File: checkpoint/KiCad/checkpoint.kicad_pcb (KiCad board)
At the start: 4 copper layers, 85.2 x 39.6 mm, 113 parts, among them J1 T0, J10 CAN_OUT, J11 BOOT, J12 Y_ENDSTOP, J13 I2C, J14 SERVO, J15 RGB, J16 SWD, J17 USB_C_Receptacle_USB2.0_16P, J18 PWR_OUT, J19 PWR_CAN_IN, J2 T1, J3 T2, J4 T3, J5 2_WIRE, J6 24_3_WIRE_A, J7 PT100, J8 23_WIRE, J9 PT100_1K, Q1 BSS138, SW1 SW_RESET, U1 MAX31865xTP, U2 SN65HVD1050D, U3 STM32G0B1CBTx, U4 USBLC6-2P6, U5 AMS1117-3.3, U6 TPS5430DDA, Y1 Crystal

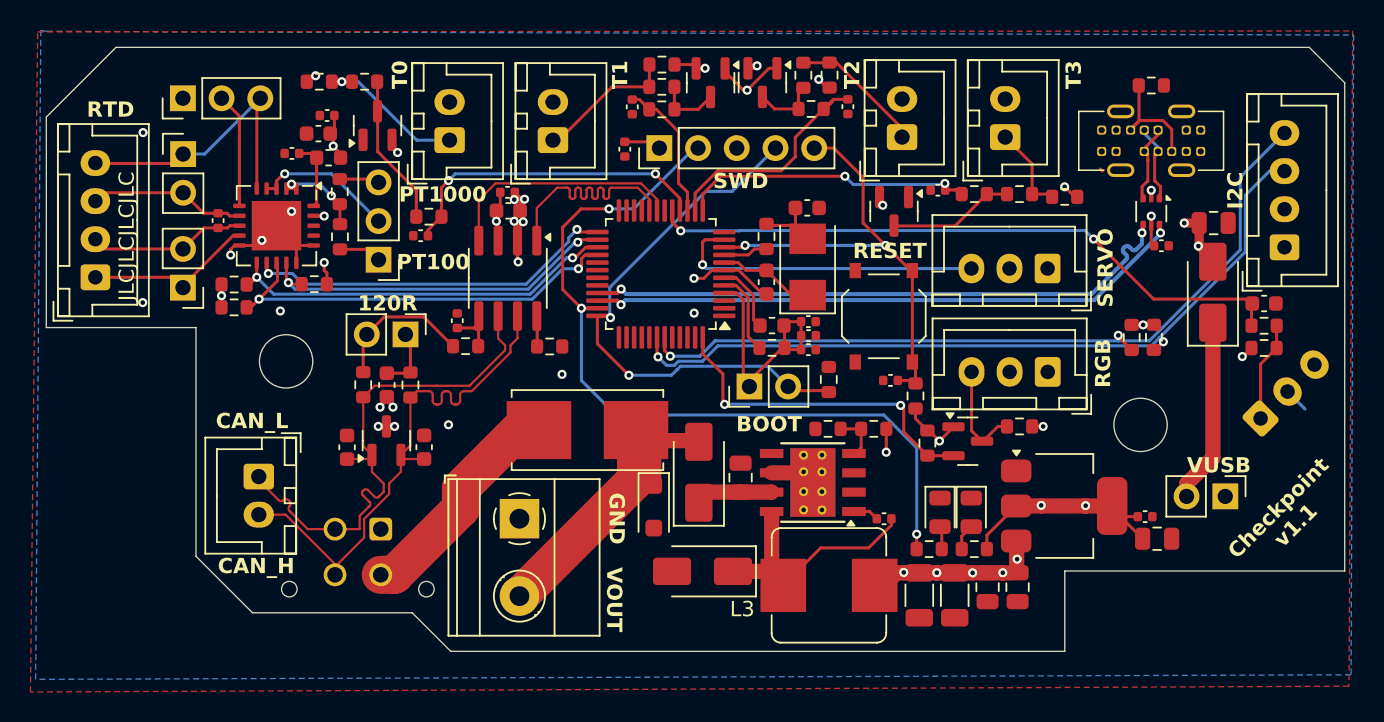
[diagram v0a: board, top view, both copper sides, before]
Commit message: chore: clean up tracks
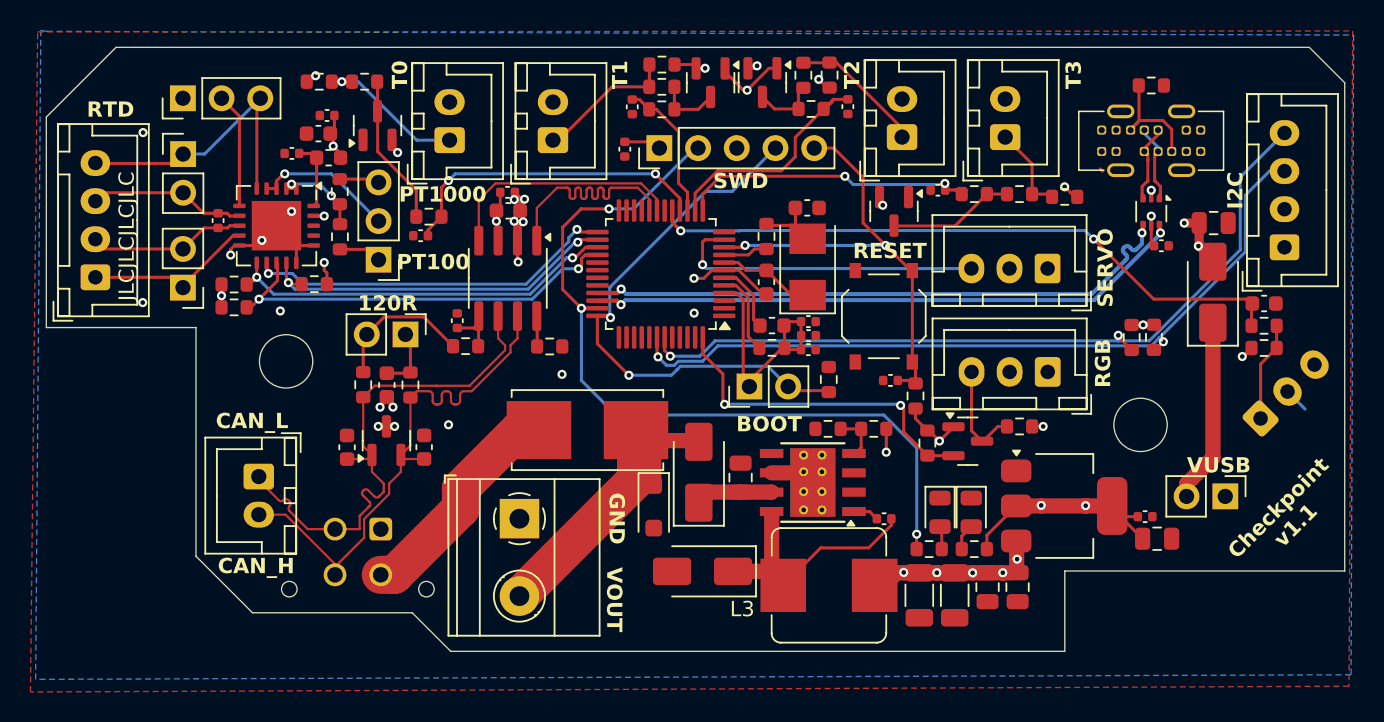
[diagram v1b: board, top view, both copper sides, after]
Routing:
- net +3.3V: track 120.7 -> 117.9 mm
- net Net-(D11-K): track 18.1 -> 15.8 mm
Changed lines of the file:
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@@
 	)
 	(segment
-		(start 44.5 57.27071)
-		(end 44.900408 57.671118)
-		(width 0.2)
-		(layer "F.Cu")
-		(net 2)
-	)
-	(segment
 		(start 53.075408 48.096118)
 		(end 53.075408 46.746118)
@@
 	)
 	(segment
+		(start 44.5 56.995)
+		(end 44.5 57.27071)
+		(width 0.2)
+		(layer "F.Cu")
+		(net 2)
+	)
+	(segment
 		(start 52.97 45.361526)
 		(end 52.97 45.066801)
@@
 	)
 	(segment
-		(start 44.5 56.995)
-		(end 44.5 57.27071)
-		(width 0.2)
-		(layer "F.Cu")
-		(net 2)
-	)
-	(segment
 		(start 53.075408 45.864592)
 		(end 53.075408 46.746118)
@@
 		(net 2)
 	)
+	(segment
+		(start 44.5 57.27071)
+		(end 44.900408 57.671118)
+		(width 0.2)
+		(layer "F.Cu")
+		(net 2)
+	)
 	(via
 		(at 34.25 47.69)
@@
 	)
 	(segment
-		(start 92.920408 65.121118)
-		(end 92.920408 63.751118)
-		(width 0.2)
-		(layer "F.Cu")
-		(net 6)
-	)
-	(segment
 		(start 85.81 64.16)
 		(end 87.411526 64.16)
@@
 	)
 	(segment
-		(start 39.440408 36.311118)
-		(end 39.245408 36.311118)
-		(width 0.2)
-		(layer "F.Cu")
-		(net 6)
-	)
-	(segment
 		(start 45.014187 40.764897)
 		(end 45.014187 40.125926)
@@
 	)
 	(segment
-		(start 89.650408 43.871118)
-		(end 89.815408 43.871118)
-		(width 0.2)
-		(layer "F.Cu")
-		(net 6)
-	)
-	(segment
 		(start 40.390408 48.691118)
 		(end 40.565408 48.866118)
@@
 	)
 	(segment
-		(start 92.811118 64.861118)
-		(end 92.11 64.16)
-		(width 0.2)
-		(layer "F.Cu")
-		(net 6)
-	)
-	(segment
 		(start 64.547908 35.188618)
 		(end 64.800408 35.441118)
@@
 	)
 	(segment
-		(start 94.840408 52.276118)
-		(end 94.850408 52.266118)
-		(width 0.2)
-		(layer "F.Cu")
-		(net 6)
-	)
-	(segment
 		(start 66.6475 50.1825)
 		(end 67.454962 50.1825)
@@
 	)
 	(segment
-		(start 38.613713 64.988713)
+		(start 38.114902 64.489903)
 		(end 39.305 65.68)
 		(width 0.1486)
@@
 	)
 	(segment
-		(start 36.095408 62.231118)
-		(end 36.095408 62.470408)
-		(width 0.1486)
-		(layer "F.Cu")
-		(net 13)
-	)
-	(segment
 		(start 39.305 65.68)
 		(end 41.1 65.68)
@@
 	)
 	(segment
-		(start 38.114902 64.489903)
-		(end 38.194099 64.569099)
-		(width 0.1486)
-		(layer "F.Cu")
-		(net 13)
-	)
-	(segment
-		(start 38.194099 64.569099)
-		(end 38.613713 64.988713)
-		(width 0.1486)
-		(layer "F.Cu")
-		(net 13)
-	)
-	(segment
 		(start 38.117755 64.170265)
 		(end 38.114902 64.173119)
@@
 	)
 	(segment
-		(start 43.89 36.335)
-		(end 43.865 36.31)
-		(width 0.2)
-		(layer "F.Cu")
-		(net 18)
-	)
-	(segment
 		(start 46.435408 43.435408)
 		(end 43.9 40.9)
@@
 		(net 24)
 	)
-	(segment
-		(start 42.213882 36.311118)
-		(end 42.215 36.31)
-		(width 0.2)
-		(layer "F.Cu")
-		(net 24)
-	)
 	(via
 		(at 41.550408 36.311118)
@@
 	)
 	(segment
-		(start 94.220408 40.891118)
-		(end 94.220408 40.691117)
-		(width 0.2)
-		(layer "F.Cu")
-		(net 63)
-	)
-	(segment
 		(start 94.074999 43.188232)
 		(end 94.42647 42.836761)
@@
 	)
 	(segment
-		(start 94.935408 53.916118)
-		(end 94.850408 53.916118)
-		(width 0.2)
-		(layer "F.Cu")
-		(net 68)
-	)
-	(segment
 		(start 62.235 54.307478)
 		(end 62.235 53.095)
@@
 	)
 	(segment
-		(start 98.720408 52.311118)
-		(end 98.540408 52.131118)
-		(width 1)
-		(layer "F.Cu")
-		(net 74)
-	)
-	(segment
 		(start 96.993862 62.717664)
 		(end 98.720408 60.991118)
@@
 	)
 	(segment
-		(start 69.600408 68.451118)
-		(end 70.520408 69.371118)
-		(width 1)
-		(layer "F.Cu")
-		(net 75)
-	)
-	(segment
 		(start 69.76 64.8)
 		(end 69.76 68.61071)
@@
 	)
 	(segment
-		(start 69.76 68.61071)
-		(end 70.520408 69.371118)
-		(width 1)
-		(layer "F.Cu")
-		(net 75)
-	)
-	(segment
 		(start 72.980408 66.911118)
 		(end 70.520408 69.371118)
@@
 	)
 	(segment
-		(start 93.855408 36.561118)
-		(end 93.870408 36.576118)
-		(width 0.2)
-		(layer "F.Cu")
-		(net 78)
-	)
-	(segment
 		(start 93.870408 36.576118)
 		(end 93.870408 38.900566)
@@
 	(segment
 		(start 93.320408 39.450566)
-		(end 93.320408 39.491118)
-		(width 0.2)
-		(layer "F.Cu")
-		(net 78)
-	)
-	(segment
-		(start 93.320408 39.450566)
 		(end 93.909856 38.861118)
 		(width 0.2)
@@
 		(target_skew_min -0.1)
 		(tuning_mode "single")
-		(members 372452fb-1985-4f5b-8778-86ad6c45a177 3f50befc-3a8a-4e98-bb7b-eb0b68ef2263
-			3f94b837-e7de-43fc-ab11-373bf12ca2e6 42eb6b5b-3ffd-4e1e-ae88-a98e7fd85fc5
+		(members 372452fb-1985-4f5b-8778-86ad6c45a177 42eb6b5b-3ffd-4e1e-ae88-a98e7fd85fc5
 			65ef1ab8-76f8-4721-b0d3-ffc62c3cd8e2 849c9ba8-f99c-4328-adc4-834899fdc622
 			8881b552-db43-4d79-b48f-55f1766a3be2 9bcd6c47-9b0d-4d24-a42e-3aa34bd92e78

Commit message: fix: replace undersized protection diodes
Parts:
- D10: value SS34 -> SS54
- D11: value SS210 -> SS54
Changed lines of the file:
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@@
 		(sheetname "Thermistors")
 		(sheetfile "thermistors.kicad_sch")
-		(attr through_hole exclude_from_pos_files exclude_from_bom)
+		(attr through_hole exclude_from_pos_files)
 		(fp_line
 			(start -1.6 -2.75)
@@
 		(sheetname "CANBUS")
 		(sheetfile "canbus.kicad_sch")
-		(attr through_hole exclude_from_pos_files exclude_from_bom)
+		(attr through_hole exclude_from_pos_files)
 		(fp_line
 			(start -1.33 3.87)
@@
 			)
 		)
-		(property "Value" "SS34"
+		(property "Value" "SS54"
 			(at 0 2.6 -90)
 			(layer "F.Fab")
@@
 		(sheetname "Thermistors")
 		(sheetfile "thermistors.kicad_sch")
-		(attr through_hole exclude_from_pos_files exclude_from_bom)
+		(attr through_hole exclude_from_pos_files)
 		(fp_line
 			(start -1.6 -2.75)
@@
 		(sheetname "CANBUS")
 		(sheetfile "canbus.kicad_sch")
-		(attr through_hole exclude_from_pos_files exclude_from_bom)
+		(attr through_hole exclude_from_pos_files)
 		(fp_line
 			(start -2.56 3.51)
@@
 		(sheetname "Power")
 		(sheetfile "power.kicad_sch")
-		(attr through_hole exclude_from_pos_files exclude_from_bom)
+		(attr through_hole exclude_from_pos_files)
 		(fp_line
 			(start -2.84 4.9)
@@
 		(sheetname "USB")
 		(sheetfile "usb.kicad_sch")
-		(attr through_hole exclude_from_pos_files exclude_from_bom)
+		(attr through_hole exclude_from_pos_files)
 		(fp_line
 			(start -1.33 3.87)
@@
 		(sheetname "Thermistors")
 		(sheetfile "thermistors.kicad_sch")
-		(attr through_hole exclude_from_pos_files exclude_from_bom)
+		(attr through_hole exclude_from_pos_files)
 		(fp_line
 			(start 1.33 1.27)
@@
 		(sheetname "MCU")
 		(sheetfile "mcu.kicad_sch")
-		(attr through_hole exclude_from_pos_files exclude_from_bom)
+		(attr through_hole exclude_from_pos_files)
 		(fp_line
 			(start 7.56 3.51)
@@
 		(sheetname "MCU")
 		(sheetfile "mcu.kicad_sch")
-		(attr through_hole exclude_from_pos_files exclude_from_bom)
+		(attr through_hole exclude_from_pos_files)
 		(fp_line
 			(start -1.33 -1.33)
@@
 		(sheetname "Thermistors")
 		(sheetfile "thermistors.kicad_sch")
-		(attr through_hole exclude_from_pos_files exclude_from_bom)
+		(attr through_hole exclude_from_pos_files)
 		(fp_line
 			(start -1.33 -1.33)
@@
 		(sheetname "Thermistors")
 		(sheetfile "thermistors.kicad_sch")
-		(attr through_hole exclude_from_pos_files exclude_from_bom)
+		(attr through_hole exclude_from_pos_files)
 		(fp_line
 			(start -1.6 -2.75)
@@
 		(sheetname "Thermistors")
 		(sheetfile "thermistors.kicad_sch")
-		(attr through_hole exclude_from_pos_files exclude_from_bom)
+		(attr through_hole exclude_from_pos_files)
 		(fp_line
 			(start -1.33 -1.33)
@@
 		(sheetname "Power")
 		(sheetfile "power.kicad_sch")
-		(attr smd exclude_from_pos_files exclude_from_bom)
+		(attr smd exclude_from_pos_files)
 		(fp_line
 			(start -3.76 -1.95)
@@
 		(sheetname "MCU")
 		(sheetfile "mcu.kicad_sch")
-		(attr through_hole exclude_from_pos_files exclude_from_bom)
+		(attr through_hole exclude_from_pos_files)
 		(fp_line
 			(start -1.33 -1.33)
@@
 		(sheetname "MCU")
 		(sheetfile "mcu.kicad_sch")
-		(attr through_hole exclude_from_pos_files exclude_from_bom)
+		(attr through_hole exclude_from_pos_files)
 		(fp_line
 			(start 7.56 3.51)
@@
 		(sheetname "Thermistors")
 		(sheetfile "thermistors.kicad_sch")
-		(attr through_hole exclude_from_pos_files exclude_from_bom)
+		(attr through_hole exclude_from_pos_files)
 		(fp_line
 			(start -1.6 -2.75)
@@
 		(sheetname "MCU")
 		(sheetfile "mcu.kicad_sch")
-		(attr through_hole exclude_from_pos_files exclude_from_bom)
+		(attr through_hole exclude_from_pos_files)
 		(fp_line
 			(start -1.6 -2.75)
@@
 			)
 		)
-		(property "Value" "SS210"
+		(property "Value" "SS54"
 			(at 0 2.6 180)
 			(layer "F.Fab")
@@
 		(sheetname "Thermistors")
 		(sheetfile "thermistors.kicad_sch")
-		(attr through_hole exclude_from_pos_files exclude_from_bom)
+		(attr through_hole exclude_from_pos_files)
 		(fp_line
 			(start 1.33 1.27)
@@
 		(sheetname "Thermistors")
 		(sheetfile "thermistors.kicad_sch")
-		(attr through_hole exclude_from_pos_files exclude_from_bom)
+		(attr through_hole exclude_from_pos_files)
 		(fp_line
 			(start -1.6 -2.75)
@@
 		(sheetname "Power")
 		(sheetfile "power.kicad_sch")
-		(attr through_hole exclude_from_pos_files exclude_from_bom)
+		(attr through_hole exclude_from_pos_files)
 		(fp_line
 			(start 6.685 2.58)
@@
 		(sheetname "MCU")
 		(sheetfile "mcu.kicad_sch")
-		(attr through_hole exclude_from_pos_files exclude_from_bom)
+		(attr through_hole exclude_from_pos_files)
 		(fp_line
 			(start -2.559999 -9.31)
